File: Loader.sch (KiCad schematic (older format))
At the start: 43 parts, among them SW1 SW_LOADER_RESET, U8 FT232RL, U9 ATmega2560-16AU, Y1 8Mhz

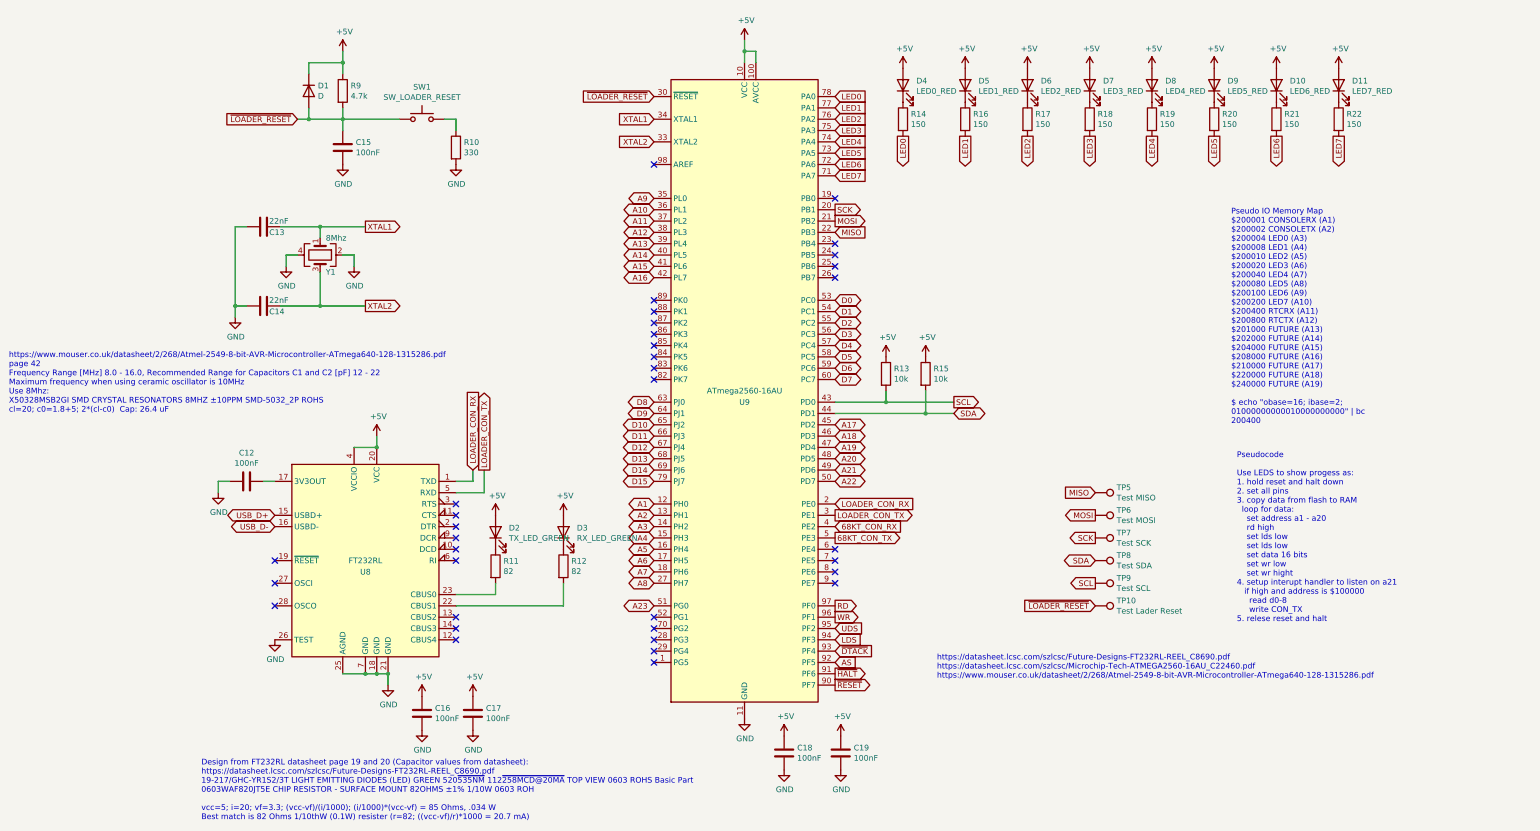
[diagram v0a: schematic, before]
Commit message: updates
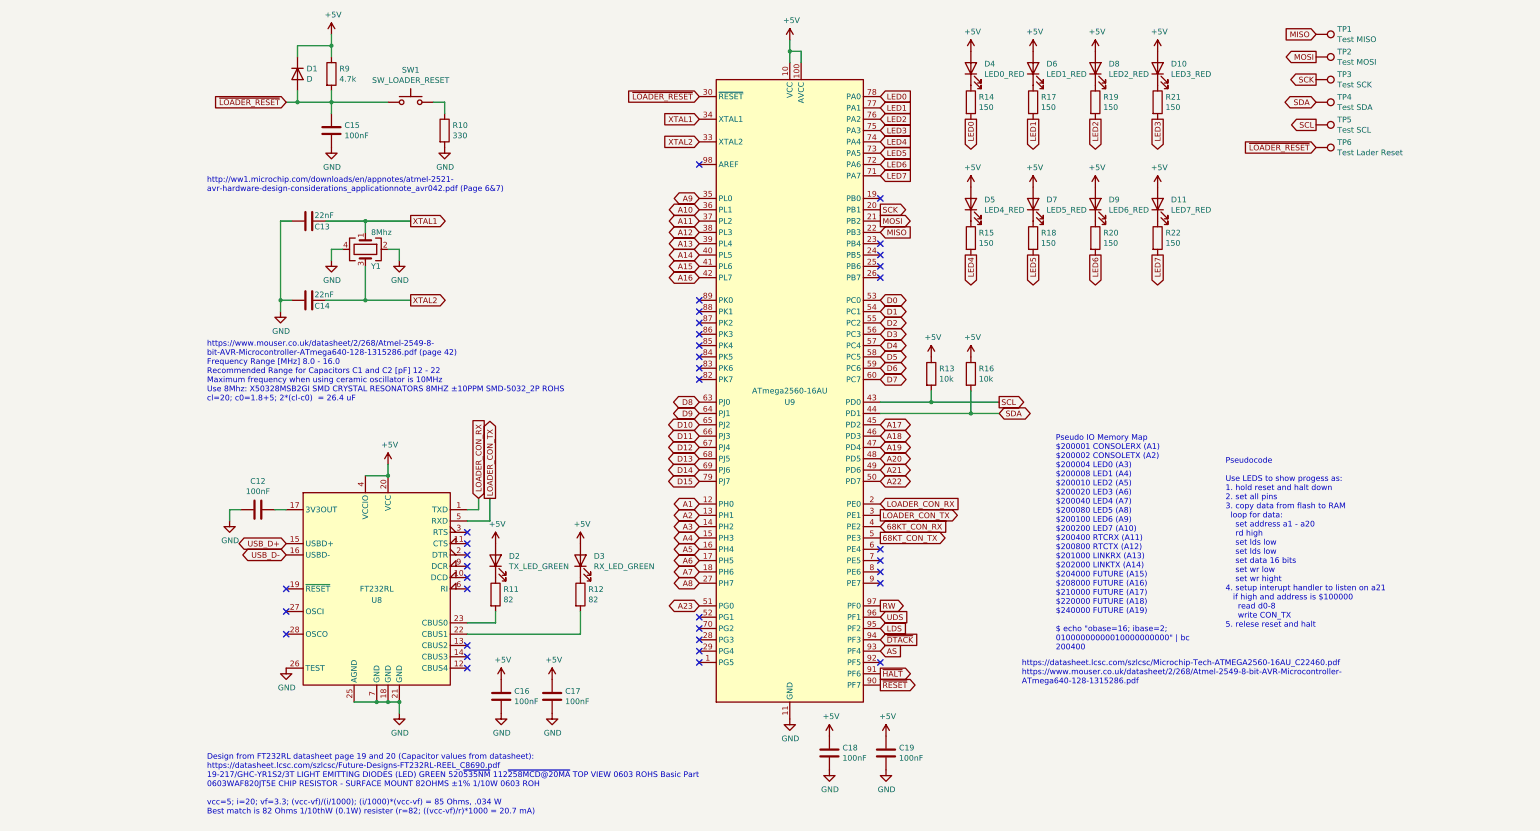
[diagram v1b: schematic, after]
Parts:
- D1: footprint (none) -> Diode_SMD:D_SMA; JLPCB Datasheet (none) -> https://datasheet.lcsc.com/szlcsc/MDD-Jiangsu-Yutai-Elec-M7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; JLPCB Part (none) -> M7
- TP1: renamed from TP5; JLPCB Datasheet (none) -> N/A; JLPCB Part (none) -> N/A
- TP2: renamed from TP6; JLPCB Datasheet (none) -> N/A; JLPCB Part (none) -> N/A
- TP3: renamed from TP7; JLPCB Datasheet (none) -> N/A; JLPCB Part (none) -> N/A
- TP4: renamed from TP8; JLPCB Datasheet (none) -> N/A; JLPCB Part (none) -> N/A
- TP5: renamed from TP9; JLPCB Datasheet (none) -> N/A; JLPCB Part (none) -> N/A
- TP6: renamed from TP10; JLPCB Datasheet (none) -> N/A; JLPCB Part (none) -> N/A
- U8: JLPCB Datasheet (none) -> https://datasheet.lcsc.com/szlcsc/Future-Designs-FT232RL-RE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; JLPCB Part (none) -> FT232RL-REEL
- renumbered D7 to D10, D8 to D5, D5 to D6, D9 to D7, D6 to D8, D10 to D9, R19 to R15, R15 to R16, R16 to R17, R20 to R18, R17 to R19, R21 to R20, R18 to R21
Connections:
- net WR is gone; now on net UDS: U9.96 (PF1)
- net AS: now also U9.93 (PF4); no longer U9.92 (PF5)
- net LDS: now also U9.95 (PF2); no longer U9.94 (PF3)
- net UDS: no longer U9.95 (PF2)
- net ~DTACK: now also U9.94 (PF3); no longer U9.93 (PF4)
- net RD renamed RW
- no-connect marks 35 -> 36
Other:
- note added: "Pseudo IO Memory Map\n$200001 CONSOLERX (A1)\n$200002 CONSOLETX (A2)\n$200004 LED0 (A3)\n$200008 LED1 (A4)\n$200010 LED2 (A5)\n$200020 LED3 (A6)\n$200040 LED4 (A7)\n$200080 LED5 (A8)\n$200100 LED6 (A9)\n$200200 LED7 (A10)\n$200400 RTCRX (A11)\n$200800 RTCTX (A12)\n$201000 LINKRX (A13)\n$202000 LINKTX (A14)\n$204000 FUTURE (A15)\n$208000 FUTURE (A16)\n$210000 FUTURE (A17)\n$220000 FUTURE (A18)\n$2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"
- note added: "http://ww1.microchip.com/downloads/en/appnotes/atmel-2521-\navr-hardware-design-considerations_applicationnote_avr042.pdf (Page 6&7)"
- note added: "https://datasheet.lcsc.com/szlcsc/Microchip-Tech-ATMEGA2560-16AU_C22460.pdf\nhttps://www.mouser.co.uk/datasheet/2/268/Atmel-2549-8-bit-AVR-Microcontroller-\nATmega640-128-1315286.pdf"
- note added: "https://www.mouser.co.uk/datasheet/2/268/Atmel-2549-8-\nbit-AVR-Microcontroller-ATmega640-128-1315286.pdf (page 42)\nFrequency Range [MHz] 8.0 - 16.0\nRecommended Range for Capacitors C1 and C2 [pF] 12 - 22\nMaximum frequency when using ceramic oscillator is 10MHz\nUse 8Mhz: X50328MSB2GI SMD CRYSTAL RESONATORS 8MHZ ±10PPM SMD-5032_2P ROHS\ncl=20; c0=1.8+5; 2*(cl-c0) = 26.4 uF\n"
- note removed: "Pseudo IO Memory Map\n$200001 CONSOLERX (A1)\n$200002 CONSOLETX (A2)\n$200004 LED0 (A3)\n$200008 LED1 (A4)\n$200010 LED2 (A5)\n$200020 LED3 (A6)\n$200040 LED4 (A7)\n$200080 LED5 (A8)\n$200100 LED6 (A9)\n$200200 LED7 (A10)\n$200400 RTCRX (A11)\n$200800 RTCTX (A12)\n$201000 FUTURE (A13)\n$202000 FUTURE (A14)\n$204000 FUTURE (A15)\n$208000 FUTURE (A16)\n$210000 FUTURE (A17)\n$220000 FUTURE (A18)\n$2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"
- note removed: "https://datasheet.lcsc.com/szlcsc/Future-Designs-FT232RL-REEL_C8690.pdf\nhttps://datasheet.lcsc.com/szlcsc/Microchip-Tech-ATMEGA2560-16AU_C22460.pdf\nhttps://www.mouser.co.uk/datasheet/2/268/Atmel-2549-8-bit-AVR-Microcontroller-ATmega640-128-1315286.pdf"
- note removed: "https://www.mouser.co.uk/datasheet/2/268/Atmel-2549-8-bit-AVR-Microcontroller-ATmega640-128-1315286.pdf\npage 42\nFrequency Range [MHz] 8.0 - 16.0, Recommended Range for Capacitors C1 and C2 [pF] 12 - 22\nMaximum frequency when using ceramic oscillator is 10MHz\nUse 8Mhz:\nX50328MSB2GI SMD CRYSTAL RESONATORS 8MHZ ±10PPM SMD-5032_2P ROHS\ncl=20; c0=1.8+5; 2*(cl-c0) Cap: 26.4 uF\n"
- moved on the sheet: C12, C13, C14, C15, C16, C17, C18, C19, D1, D10, D11, D2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

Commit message: update
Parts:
- C13, C14: footprint (none) -> Capacitor_SMD:C_0603_1608Metric
- R10: footprint (none) -> Resistor_SMD:R_0603_1608Metric; JLPCB Datasheet (none) -> https://datasheet.lcsc.com/szlcsc/Uniroyal-Elec-0603WAF3300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; JLPCB Part (none) -> 0603WAF3300T5E
- R13, R16: footprint (none) -> Resistor_SMD:R_0603_1608Metric; JLPCB Datasheet (none) -> https://datasheet.lcsc.com/szlcsc/Uniroyal-Elec-0603WAF1002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; JLPCB Part (none) -> 0603WAF1002T5E
- R9: footprint (none) -> Resistor_SMD:R_0603_1608Metric; JLPCB Datasheet (none) -> https://datasheet.lcsc.com/szlcsc/Uniroyal-Elec-0603WAF4701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; JLPCB Part (none) -> 0603WAF4701T5E
- SW1: footprint (none) -> Button_Switch_SMD:SW_Push_1P1T_NO_6x6mm_H9.5mm; JLPCB Datasheet (none) -> https://datasheet.lcsc.com/szlcsc/2006230332_USAKRO-UK-B022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; JLPCB Part (none) -> UK-B0228-G5-160-JZ
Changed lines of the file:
@@
 F 0 "R16" H 7370 3796 50  0000 L CNN
 F 1 "10k" H 7370 3705 50  0000 L CNN
-F 2 "" V 7230 3750 50  0001 C CNN
+F 2 "Resistor_SMD:R_0603_1608Metric" V 7230 3750 50  0001 C CNN
 F 3 "~" H 7300 3750 50  0001 C CNN
+F 4 "https://datasheet.lcsc.com/szlcsc/Uniroyal-Elec-0603WAF1002T5E_C25804.pdf" H 7300 3750 50  0001 C CNN "JLPCB Datasheet"
+F 5 "0603WAF1002T5E" H 7300 3750 50  0001 C CNN "JLPCB Part"
 	1    7300 3750
 	1    0    0    -1
@@
 F 0 "R13" H 7020 3796 50  0000 L CNN
 F 1 "10k" H 7020 3705 50  0000 L CNN
-F 2 "" V 6880 3750 50  0001 C CNN
+F 2 "Resistor_SMD:R_0603_1608Metric" V 6880 3750 50  0001 C CNN
 F 3 "~" H 6950 3750 50  0001 C CNN
+F 4 "https://datasheet.lcsc.com/szlcsc/Uniroyal-Elec-0603WAF1002T5E_C25804.pdf" H 6950 3750 50  0001 C CNN "JLPCB Datasheet"
+F 5 "0603WAF1002T5E" H 6950 3750 50  0001 C CNN "JLPCB Part"
 	1    6950 3750
 	1    0    0    -1
@@
 F 0 "SW1" H 2350 1635 50  0000 C CNN
 F 1 "SW_LOADER_RESET" H 2350 1544 50  0000 C CNN
-F 2 "" H 2350 1550 50  0001 C CNN
+F 2 "Button_Switch_SMD:SW_Push_1P1T_NO_6x6mm_H9.5mm" H 2350 1550 50  0001 C CNN
 F 3 "~" H 2350 1550 50  0001 C CNN
+F 4 "https://datasheet.lcsc.com/szlcsc/2006230332_USAKRO-UK-B0228-G5-160-JZ_C620316.pdf" H 2350 1350 50  0001 C CNN "JLPCB Datasheet"
+F 5 "UK-B0228-G5-160-JZ " H 2350 1350 50  0001 C CNN "JLPCB Part"
 	1    2350 1350
 	1    0    0    -1
@@
 F 0 "R9" H 1720 1146 50  0000 L CNN
 F 1 "4.7k" H 1720 1055 50  0000 L CNN
-F 2 "" V 1580 1100 50  0001 C CNN
+F 2 "Resistor_SMD:R_0603_1608Metric" V 1580 1100 50  0001 C CNN
 F 3 "~" H 1650 1100 50  0001 C CNN
+F 4 "https://datasheet.lcsc.com/szlcsc/Uniroyal-Elec-0603WAF4701T5E_C23162.pdf" H 1650 1100 50  0001 C CNN "JLPCB Datasheet"
+F 5 "0603WAF4701T5E " H 1650 1100 50  0001 C CNN "JLPCB Part"
 	1    1650 1100
 	1    0    0    -1
@@
 F 0 "R10" H 2720 1646 50  0000 L CNN
 F 1 "330" H 2720 1555 50  0000 L CNN
-F 2 "" V 2580 1600 50  0001 C CNN
+F 2 "Resistor_SMD:R_0603_1608Metric" V 2580 1600 50  0001 C CNN
 F 3 "~" H 2650 1600 50  0001 C CNN
+F 4 "https://datasheet.lcsc.com/szlcsc/Uniroyal-Elec-0603WAF3300T5E_C23138.pdf" H 2650 1600 50  0001 C CNN "JLPCB Datasheet"
+F 5 "0603WAF3300T5E" H 2650 1600 50  0001 C CNN "JLPCB Part"
 	1    2650 1600
 	1    0    0    -1
@@
 F 0 "C13" V 1400 2350 50  0000 R CNN
 F 1 "22nF" V 1500 2350 50  0000 R CNN
-F 2 "" H 1488 2250 50  0001 C CNN
+F 2 "Capacitor_SMD:C_0603_1608Metric" H 1488 2250 50  0001 C CNN
 F 3 "~" H 1450 2400 50  0001 C CNN
 	1    1450 2400
@@
 F 0 "C14" V 1400 3050 50  0000 R CNN
 F 1 "22nF" V 1500 3050 50  0000 R CNN
-F 2 "" H 1488 2950 50  0001 C CNN
+F 2 "Capacitor_SMD:C_0603_1608Metric" H 1488 2950 50  0001 C CNN
 F 3 "~" H 1450 3100 50  0001 C CNN
 	1    1450 3100
